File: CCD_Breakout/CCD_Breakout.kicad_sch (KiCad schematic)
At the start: 10 parts, among them J1 Conn_01x03_Pin, U1 ILX511

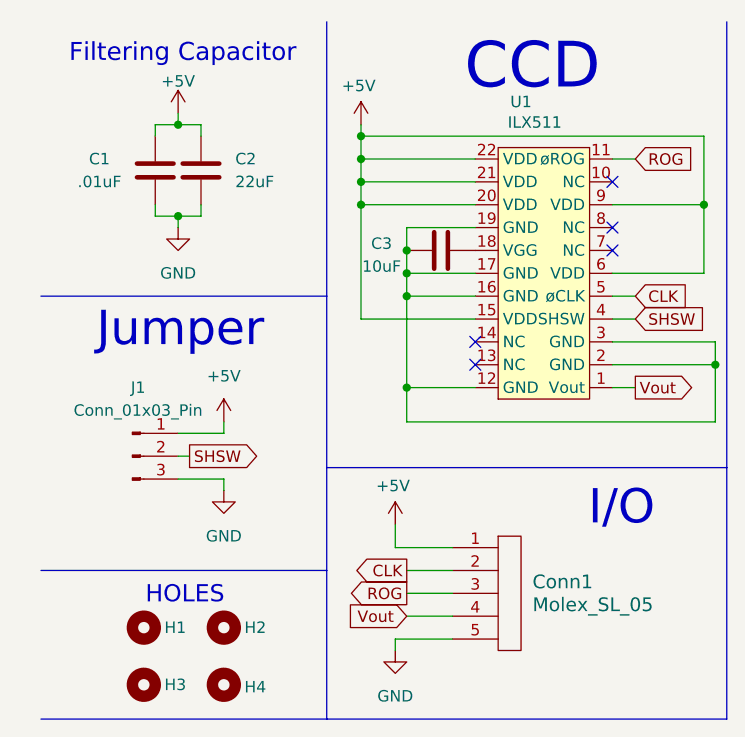
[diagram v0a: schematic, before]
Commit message: CCD GND
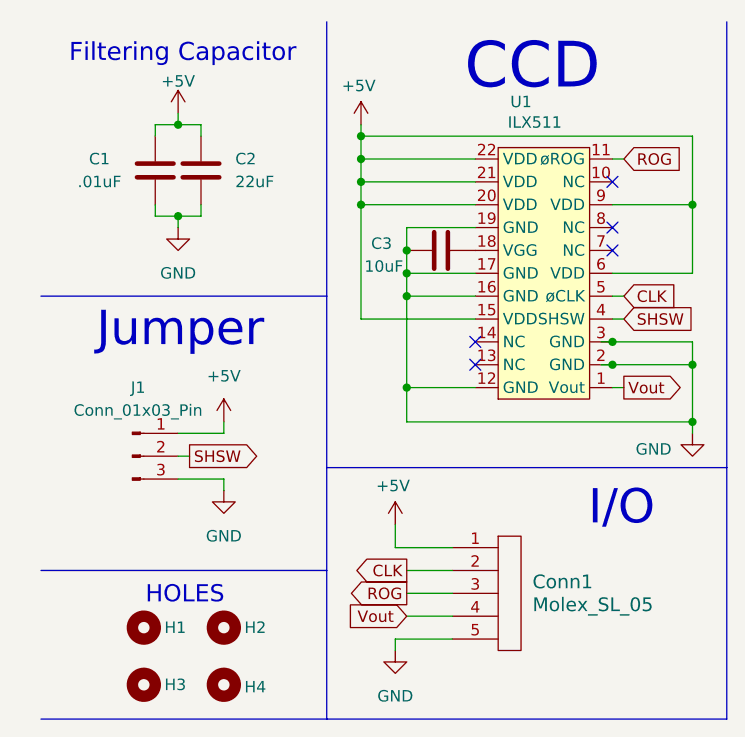
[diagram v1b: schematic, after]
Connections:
- net GND: now also C3.1, U1.12 (GND), U1.16 (GND), U1.17 (GND), U1.19 (GND), U1.2 (GND), U1.3 (GND)
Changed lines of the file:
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@@
+	)
+	(junction
+		(at 74.93 46.99)
+		(diameter 0)
+		(color 0 0 0 0)
 	)
 	(junction
@@
 	)
 	(junction
-		(at 86.36 49.53)
+		(at 83.82 49.53)
 		(diameter 0)
 		(color 0 0 0 0)
 	)
 	(junction
-		(at 85.09 31.75)
+		(at 83.82 31.75)
 		(diameter 0)
 		(color 0 0 0 0)
@@
 		(color 0 0 0 0)
 	)
+	(junction
+		(at 83.82 55.88)
+		(diameter 0)
+		(color 0 0 0 0)
+	)
+	(junction
+		(at 74.93 49.53)
+		(diameter 0)
+		(color 0 0 0 0)
+	)
 	(no_connect
 		(at 59.69 49.53)
@@
 	(wire
 		(pts
-			(xy 74.93 31.75) (xy 85.09 31.75)
+			(xy 74.93 31.75) (xy 83.82 31.75)
 		)
 		(stroke
@@
 	(wire
 		(pts
+			(xy 83.82 55.88) (xy 83.82 57.15)
+		)
+		(stroke
+			(width 0)
+			(type default)
+		)
+	)
+	(wire
+		(pts
 			(xy 57.15 69.85) (xy 50.8 69.85)
 		)
@@
 	(wire
 		(pts
-			(xy 86.36 49.53) (xy 86.36 55.88)
+			(xy 83.82 49.53) (xy 83.82 55.88)
 		)
 		(stroke
@@
 	(wire
 		(pts
-			(xy 46.99 24.13) (xy 85.09 24.13)
+			(xy 46.99 24.13) (xy 83.82 24.13)
 		)
 		(stroke
@@
 		)
 	)
+	(wire
+		(pts
+			(xy 73.66 49.53) (xy 74.93 49.53)
+		)
+		(stroke
+			(width 0)
+			(type default)
+		)
+	)
 	(polyline
 		(pts
@@
 	(wire
 		(pts
-			(xy 74.93 46.99) (xy 86.36 46.99)
-		)
-		(stroke
-			(width 0)
-			(type default)
-		)
-	)
-	(wire
-		(pts
-			(xy 85.09 31.75) (xy 85.09 24.13)
+			(xy 83.82 31.75) (xy 83.82 24.13)
 		)
 		(stroke
@@
 	(wire
 		(pts
-			(xy 86.36 55.88) (xy 52.07 55.88)
+			(xy 83.82 55.88) (xy 52.07 55.88)
 		)
 		(stroke
@@
 	(wire
 		(pts
-			(xy 74.93 41.91) (xy 77.47 41.91)
+			(xy 74.93 46.99) (xy 83.82 46.99)
+		)
+		(stroke
+			(width 0)
+			(type default)
+		)
+	)
+	(wire
+		(pts
+			(xy 73.66 46.99) (xy 74.93 46.99)
+		)
+		(stroke
+			(width 0)
+			(type default)
+		)
+	)
+	(wire
+		(pts
+			(xy 74.93 41.91) (xy 76.2 41.91)
 		)
 		(stroke
@@
 	(wire
 		(pts
-			(xy 74.93 52.07) (xy 77.47 52.07)
-		)
-		(stroke
-			(width 0)
-			(type default)
-		)
-	)
-	(wire
-		(pts
-			(xy 86.36 49.53) (xy 74.93 49.53)
+			(xy 74.93 52.07) (xy 76.2 52.07)
+		)
+		(stroke
+			(width 0)
+			(type default)
+		)
+	)
+	(wire
+		(pts
+			(xy 83.82 49.53) (xy 74.93 49.53)
 		)
 		(stroke
@@
 	(wire
 		(pts
-			(xy 74.93 26.67) (xy 77.47 26.67)
+			(xy 74.93 26.67) (xy 76.2 26.67)
 		)
 		(stroke
@@
 	(wire
 		(pts
-			(xy 74.93 44.45) (xy 77.47 44.45)
+			(xy 74.93 44.45) (xy 76.2 44.45)
 		)
 		(stroke
@@
 	(wire
 		(pts
-			(xy 85.09 39.37) (xy 85.09 31.75)
-		)
-		(stroke
-			(width 0)
-			(type default)
-		)
-	)
-	(wire
-		(pts
-			(xy 74.93 39.37) (xy 85.09 39.37)
+			(xy 83.82 39.37) (xy 83.82 31.75)
+		)
+		(stroke
+			(width 0)
+			(type default)
+		)
+	)
+	(wire
+		(pts
+			(xy 74.93 39.37) (xy 83.82 39.37)
 		)
 		(stroke
@@
 	(wire
 		(pts
-			(xy 86.36 46.99) (xy 86.36 49.53)
+			(xy 83.82 46.99) (xy 83.82 49.53)
 		)
 		(stroke
@@
 	(global_label "CLK"
 		(shape input)
-		(at 77.47 41.91 0)
+		(at 76.2 41.91 0)
 		(fields_autoplaced yes)
 		(effects
@@
 		)
 		(property "Intersheetrefs" "${INTERSHEET_REFS}"
-			(at 84.0233 41.91 0)
+			(at 82.7533 41.91 0)
 			(effects
 				(font
@@
 	(global_label "ROG"
 		(shape input)
-		(at 77.47 26.67 0)
+		(at 76.2 26.67 0)
 		(fields_autoplaced yes)
 		(effects
@@
 		)
 		(property "Intersheetrefs" "${INTERSHEET_REFS}"
-			(at 84.3257 26.67 0)
+			(at 83.0557 26.67 0)
 			(effects
 				(font
@@
 	(global_label "SHSW"
 		(shape input)
-		(at 77.47 44.45 0)
+		(at 76.2 44.45 0)
 		(fields_autoplaced yes)
 		(effects
@@
 		)
 		(property "Intersheetrefs" "${INTERSHEET_REFS}"
-			(at 85.6561 44.45 0)
+			(at 84.3861 44.45 0)
 			(effects
 				(font
@@
 	(global_label "Vout"
 		(shape output)
-		(at 77.47 52.07 0)
+		(at 76.2 52.07 0)
 		(fields_autoplaced yes)
 		(effects
@@
 		)
 		(property "Intersheetrefs" "${INTERSHEET_REFS}"
-			(at 84.5675 52.07 0)
+			(at 83.2975 52.07 0)
 			(effects
 				(font
@@
 		)
 		(property "Value" "10uF"
-			(at 49.276 38.608 90)
+			(at 49.53 38.608 90)
 			(effects
 				(font
@@
 					(unit 1)
 				)
+			)
+		)
+	)
+	(symbol
+		(lib_id "power:GND")
+		(at 83.82 57.15 0)
+		(unit 1)
+		(exclude_from_sim no)
+		(in_bom yes)
+		(on_board yes)
+		(dnp no)
+		(property "Reference" "#PWR08"
+			(at 83.82 63.5 0)
+			(effects
+				(font
+					(size 1.27 1.27)
+				)
+				(hide yes)
+			)
+		)
+		(property "Value" "GND"
+			(at 79.502 58.928 0)
+			(effects
+				(font
+					(size 1.27 1.27)
+				)
+			)
+		)
+		(property "Footprint" ""
+			(at 83.82 57.15 0)
+			(effects
+				(font
+					(size 1.27 1.27)
+				)
+				(hide yes)
+			)
+		)
+		(property "Datasheet" ""
+			(at 83.82 57.15 0)
+			(effects
+				(font
+					(size 1.27 1.27)
+				)
+				(hide yes)
+			)
+		)
+		(property "Description" "Power symbol creates a global label with name \"GND\" , ground"
+			(at 83.82 57.15 0)
+			(effects
+				(font
+					(size 1.27 1.27)
+				)
+				(hide yes)
+			)
+		)
+		(pin "1"
+		)
+		(instances
+			(project "CCD_Breakout"
+				(path "/8c44394f-ce06-4603-9f88-0202e05c26c7"
+					(reference "#PWR08")
+					(unit 1)
+				)
